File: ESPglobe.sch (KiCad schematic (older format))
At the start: 8 parts, among them P1 ESP-01, P2 TXRX, P3 PWR, P4 GPIO, U1 LD1117

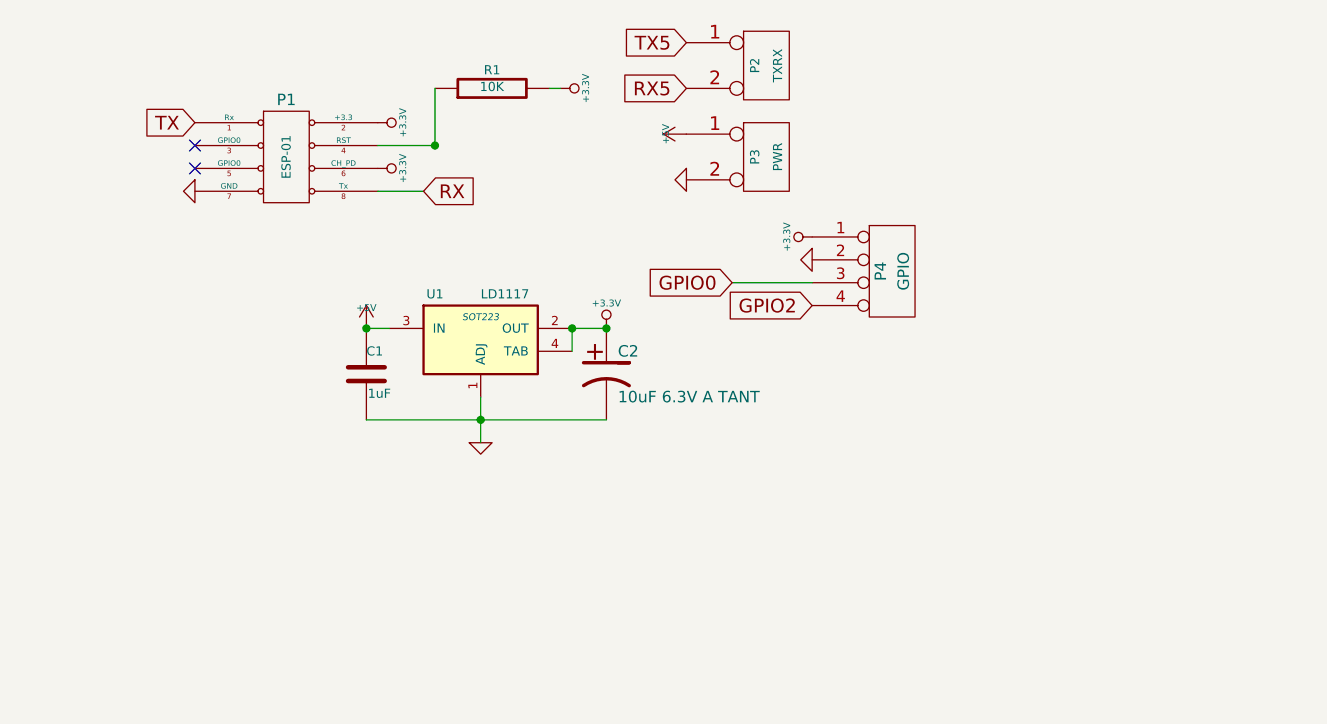
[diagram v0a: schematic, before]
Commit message: PCB design complete
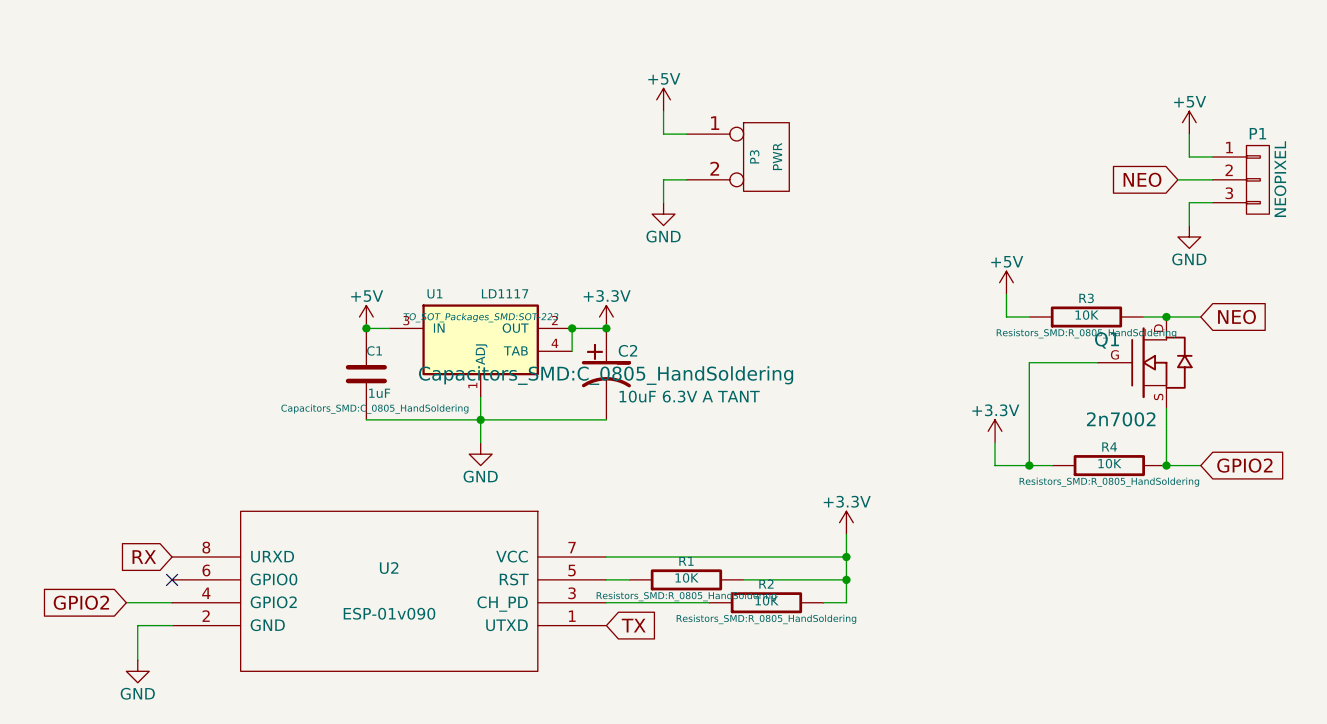
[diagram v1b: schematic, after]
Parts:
- removed P1: ESP-01, symbol ESP-01
- removed P2: TXRX, symbol CONN_2
- removed P4: GPIO, symbol CONN_4
- added P1: NEOPIXEL, Pin_Headers:Pin_Header_Straight_1x03, symbol CONN_01X03
- added Q1: 2n7002, FT:SOT23_FET, symbol MOSFET_N
- added R2, R3, R4: 10K, Resistors_SMD:R_0805_HandSoldering, symbol R-RESCUE-ESPglobe
- added U2: ESP-01v090, Pin_Headers:Pin_Header_Straight_2x04, symbol ESP-01v090
- C1, C2: footprint ~ -> Capacitors_SMD:C_0805_HandSoldering
- P3: footprint (none) -> Pin_Headers:Pin_Header_Angled_1x02
- R1: footprint ~ -> Resistors_SMD:R_0805_HandSoldering
- U1: footprint SOT223 -> TO_SOT_Packages_SMD:SOT-223
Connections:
- net +5V: now also P1.1 (P1), R3.1
- net GND: now also P1.3 (P3), U2.2 (GND)
- net GPIO2: now also Q1.S, R4.2, U2.4 (GPIO2)
- net RX: now also U2.8 (URXD)
- net TX: now also U2.1 (UTXD)
- net at R1.1: now also U2.5 (RST)
- net +3.3V renamed +3V3
- net +3V3: now also Q1.G, R2.2, R4.1, U2.7 (VCC)
- new net: R2.1, U2.3 (CH_PD)
- new net NEO: P1.2 (P2), Q1.D, R3.2
- no-connect marks 2 -> 1
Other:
- moved on the sheet: R1
